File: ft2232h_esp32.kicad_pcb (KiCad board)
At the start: 4 copper layers, 21.8 x 49.3 mm, 72 parts, among them J1 USB_C_Receptacle_USB2.0, Q1 S8050, Q2 S8050, SW1 SW_SPDT, U1 ESP32FullConnector, U10 USBLC6-2SC6-Power_Protection, U11 USBLC6-2SC6-Power_Protection, U12 USBLC6-2SC6-Power_Protection, U13 USBLC6-2SC6-Power_Protection, U2 ESP32FullConnector, U3 USBLC6-2SC6-Power_Protection, U4 93C56-C173182, U5 FT2232HL, U8 XC6206P332MR, U9 SY8089AAAC, X1 ASCO

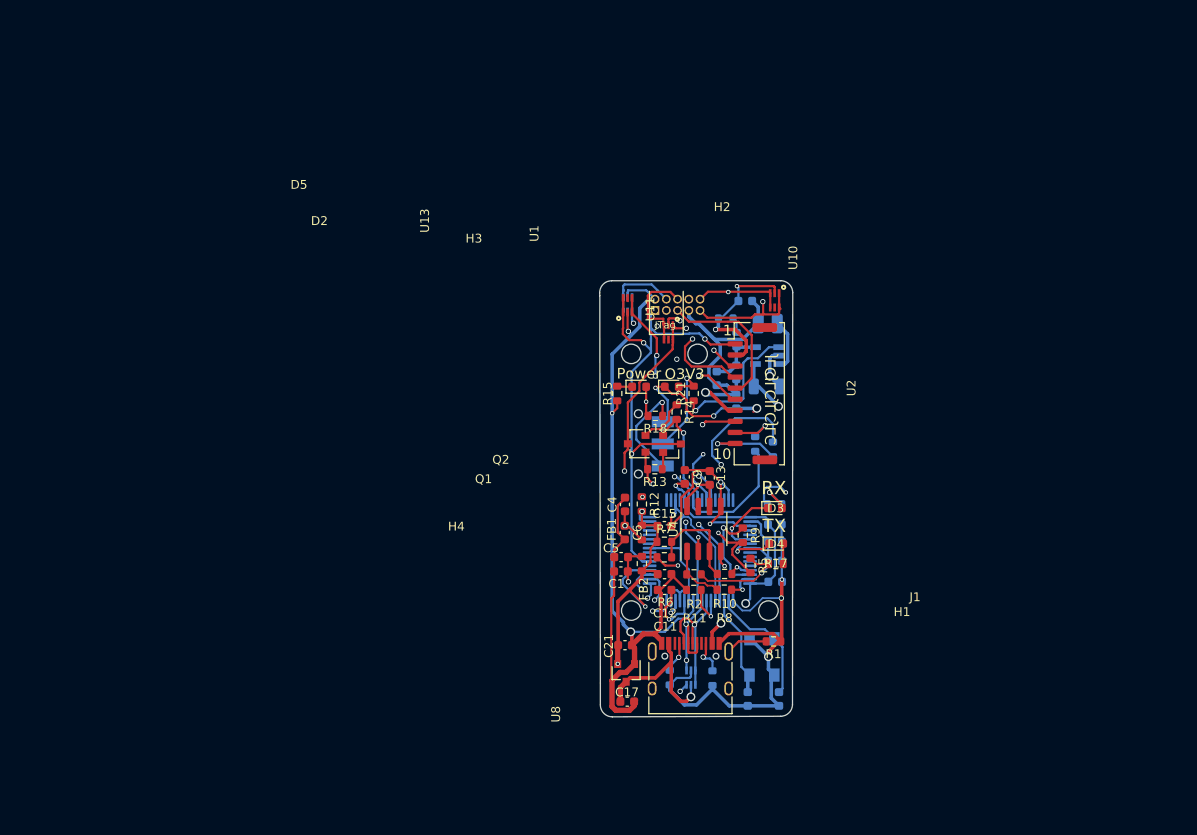
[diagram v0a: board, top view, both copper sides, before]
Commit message: V0
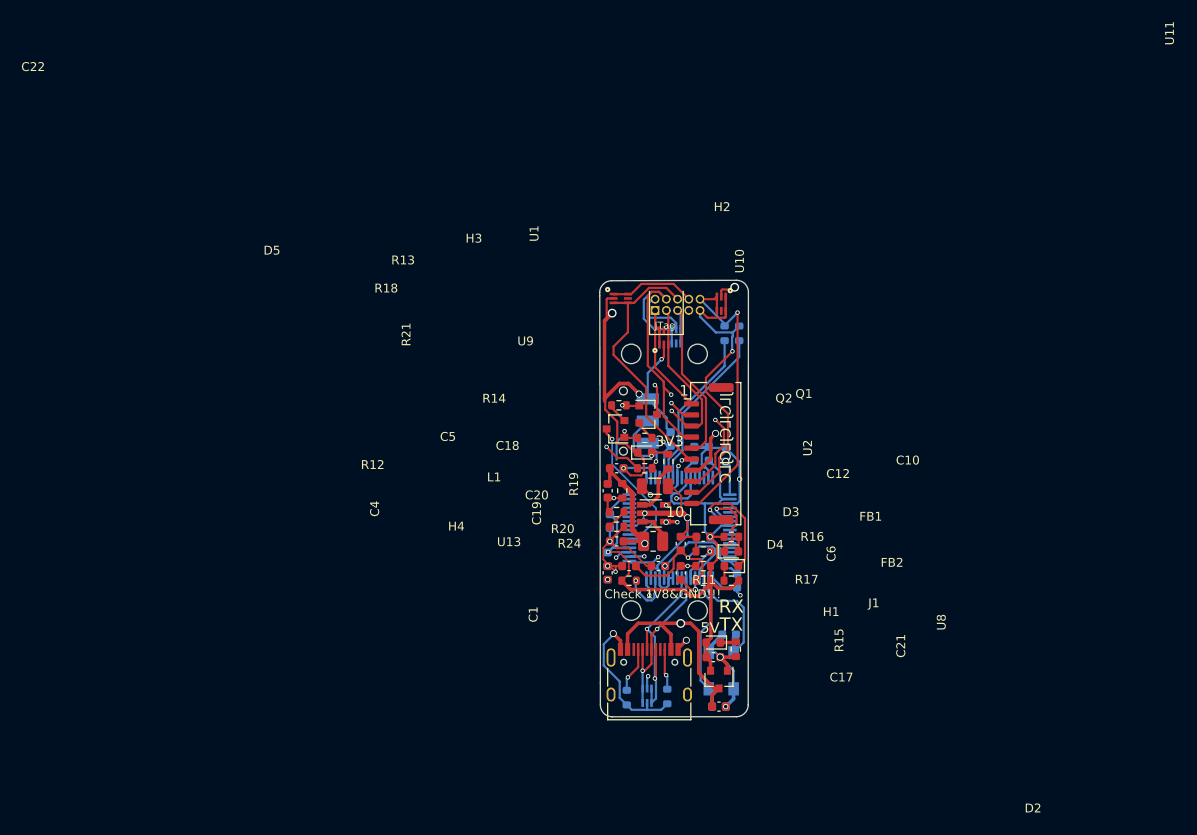
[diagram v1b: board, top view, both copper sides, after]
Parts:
- removed R1: 0, Resistor_SMD:R_0603_1608Metric
- removed R10, R8, R9: 33R(1%), Resistor_SMD:R_0603_1608Metric
- removed R2, R5, R7: 10k(1%), Resistor_SMD:R_0603_1608Metric
- removed R6: 2.2k(1%), Resistor_SMD:R_0603_1608Metric
- removed U4: 93C56-C173182, Package_SO:SOP-8_3.76x4.96mm_P1.27mm
- C10, C18, C19, C20, C22, L1, R16, R19, R20, R24, U9: moved to F.Cu
- C11, C13, C15, C9: moved to B.Cu
- moved R15 31.8 mm to (120.7, 89.7)
- moved C20 30.8 mm to (107.2, 77.5)
- moved D2 30.1 mm to (118.1, 88.9), turned to 180 degrees
- moved L1 27.8 mm to (111.3, 77.5)
- moved R24 26.6 mm to (107.2, 75.8), turned to 0 degrees
- moved R20 23.7 mm to (107.2, 74.2), turned to 180 degrees
- moved U9 21.9 mm to (111.4, 74.3), turned to 0 degrees
- moved R19 18.6 mm to (107.8, 71.8), turned to 90 degrees
- moved C19 17.7 mm to (106.2, 71.8), turned to 270 degrees
- moved C11 17.1 mm to (113.3, 65.9), turned to 90 degrees
- moved C22 16.9 mm to (111.5, 71.2)
- moved C18 15.5 mm to (107.2, 69.2), turned to 180 degrees
- moved C14 15.2 mm to (116.0, 67.6), turned to 90 degrees
- moved C13 14.7 mm to (106.2, 79.5), turned to 270 degrees
- moved R22 14.2 mm to (119.4, 54.0), turned to 270 degrees
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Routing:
- net +3V3: track 130.3 -> 92.4 mm, vias 8 -> 3
- net GND: track 314.8 -> 282.2 mm, vias 17 -> 18
- net 3v3OUT: track 34.2 -> 62.9 mm, vias 1 -> 2
- net Net-(R12-Pad1): track 29.3 -> 5.98 mm, vias 2 -> 1
- net TDO: track 65.2 -> 48.4 mm
- net TDI: track 60.0 -> 43.6 mm, vias 4 -> 2
- net TCK: track 77.1 -> 62.0 mm
- net EECLK: track 12.5 -> 0.00 mm, vias 2 -> 0
- net EEDATA: track 11.9 -> 0.00 mm
- net nRTS: track 12.6 -> 23.9 mm, vias 1 -> 2
- net VBUS: track 65.7 -> 54.8 mm, vias 3 -> 5
- net Net-(U5-Pad62): track 10.6 -> 0.00 mm, vias 1 -> 0
- net Net-(R21-Pad1): track 16.0 -> 5.80 mm, vias 1 -> 0
- net Net-(R6-Pad2): track 9.87 -> 0.00 mm, vias 2 -> 0
- net ESPRX: track 43.5 -> 34.3 mm, vias 2 -> 1
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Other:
- board size 21.8 x 49.3 mm -> 16.8 x 49.3 mm
- board text added: "3V3"
- board text added: "5V"
- board text added: "Check 1V8&GND!!!"
- board text added: "KisonHe FT2232C-NE-V0"
- board text removed: "KisonHe FT2232C-V2"
- board text removed: "O3V3"
- board text removed: "Power"
